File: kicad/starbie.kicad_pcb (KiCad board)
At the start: 2 copper layers, 118.5 x 114.8 mm, 9 parts, among them J1 Conn_01x04_Pin, J2 Conn_01x08_Pin, SW1 SW_Push, SW2 SW_Push, U1 XIAO-ESP32-C3-SMD, U2 DHT11

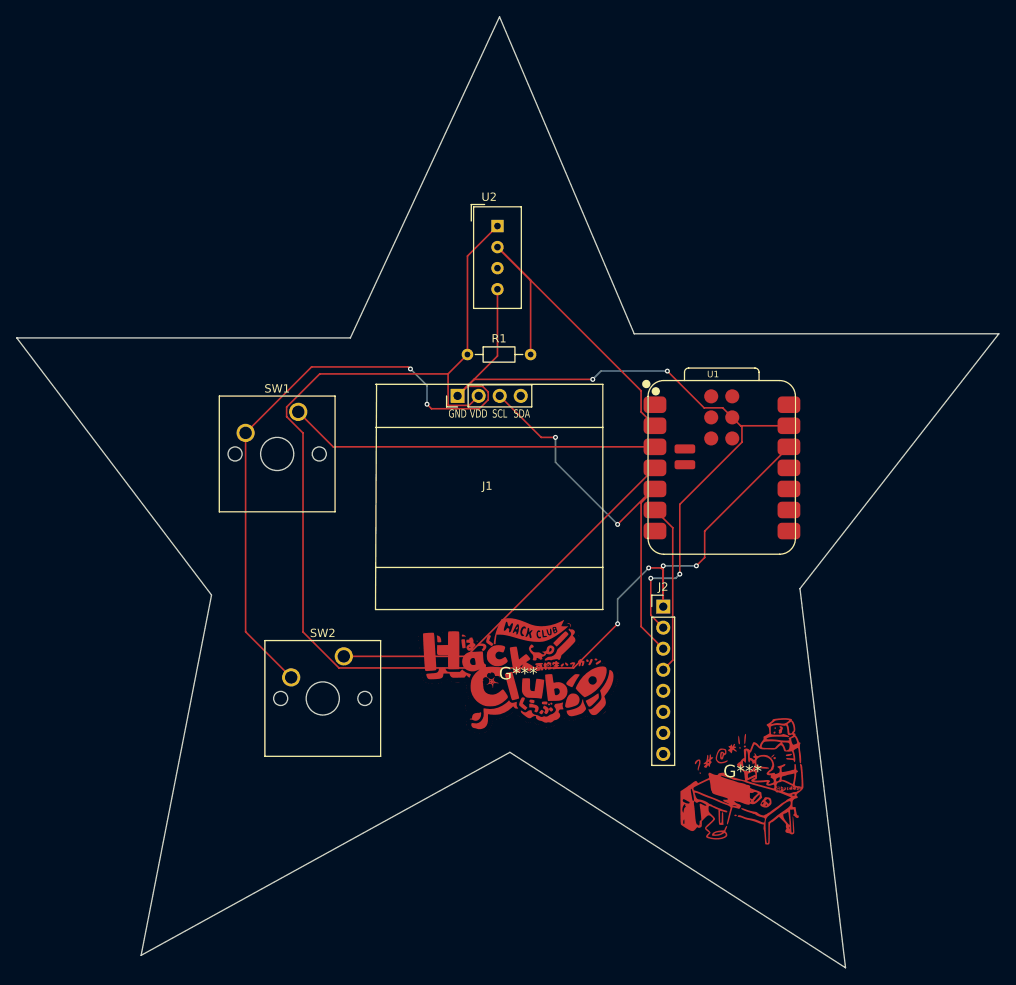
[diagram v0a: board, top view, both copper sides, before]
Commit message: pcb edit
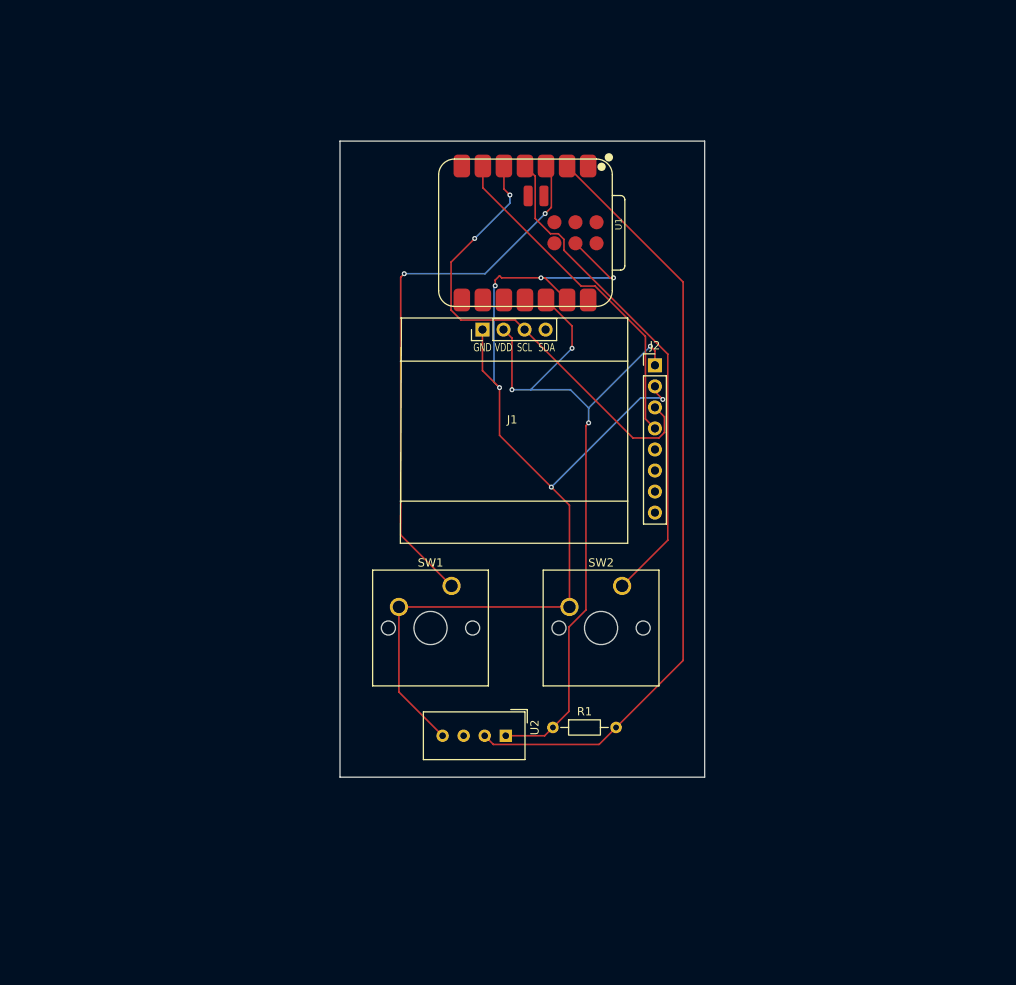
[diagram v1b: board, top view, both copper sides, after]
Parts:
- removed G***: LOGO, pcbimages:hclogo
- removed G***: LOGO, pcbimages:mad3
- moved U2 61.5 mm to (169.0, 110.0), turned to -90 degrees
- moved U1 54.1 mm to (160.8, 40.4), turned to -90 degrees
- moved R1 46.2 mm to (174.7, 109.0)
- moved SW2 34.6 mm to (183.0, 91.9)
- moved J2 29.1 mm to (187.0, 65.3)
- moved SW1 28.0 mm to (162.5, 91.9)
- moved J1 8.54 mm to (170.0, 61.0)
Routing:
- net +3.3V: track 161.8 -> 91.5 mm
- net /DHT11 DATA: track 44.0 -> 94.0 mm
- net GND: track 163.7 -> 134.6 mm
- net /GPIO2: track 44.8 -> 66.7 mm, vias 0 -> 2
- net /SDA: track 20.6 -> 41.2 mm
- net /GPIO3: track 47.0 -> 60.6 mm
- net /SCL: track 49.8 -> 56.5 mm
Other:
- board size 118.5 x 114.8 mm -> 44 x 76.8 mm
